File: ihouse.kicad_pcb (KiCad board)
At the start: 2 copper layers, 42 parts, among them J1 Conn_01x01, J2 Conn_01x01, J3 Conn_01x01, J4 Conn_01x01, J5 Conn_01x16, J6 Conn_01x02, J7 Conn_01x02, K1 FINDER-32.21-x300, K2 RT42xxxx, K3 FINDER-32.21-x300, K4 RT42xxxx, K5 G5Q-1A, K6 G5Q-1A, T1 Transformer_TEZ_22x24_6V, U1 LTV-817, U3 MOC3060S, U4 LTV-817, U5 MOC3060S

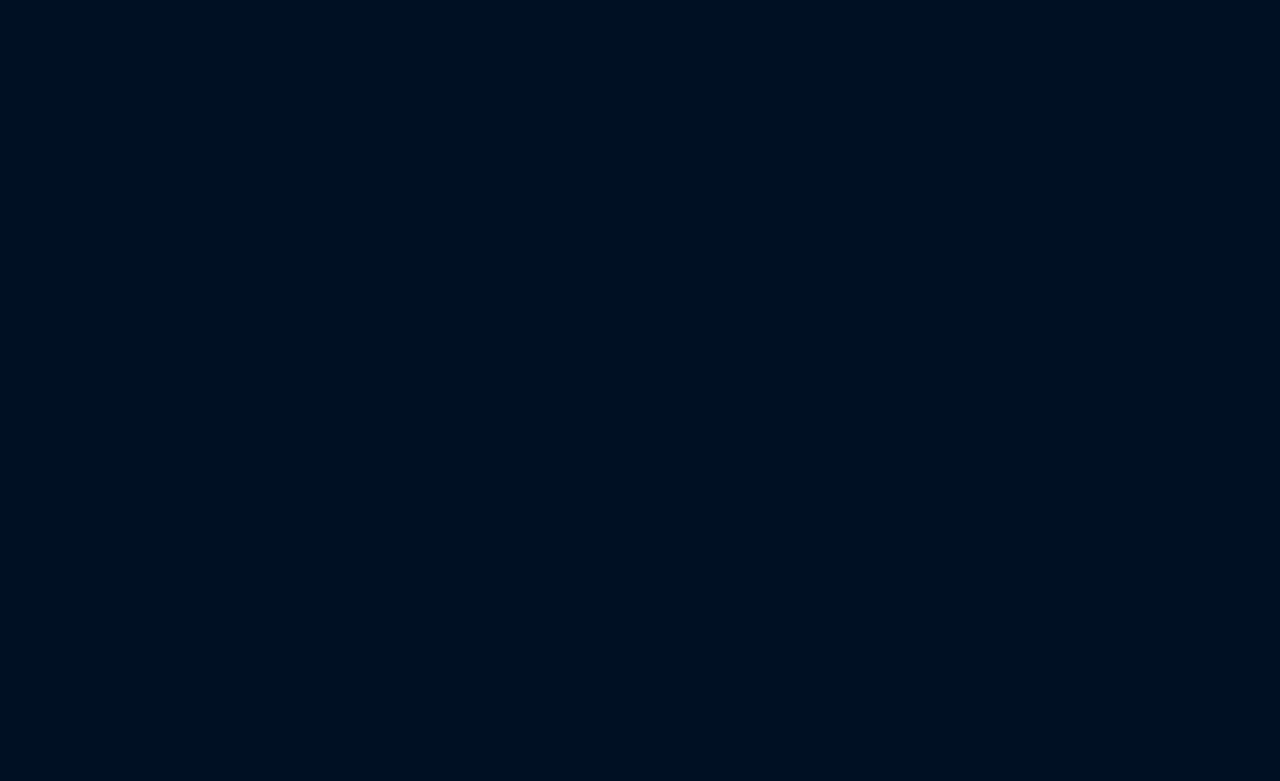
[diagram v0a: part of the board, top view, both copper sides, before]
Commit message: schemos paruosimas
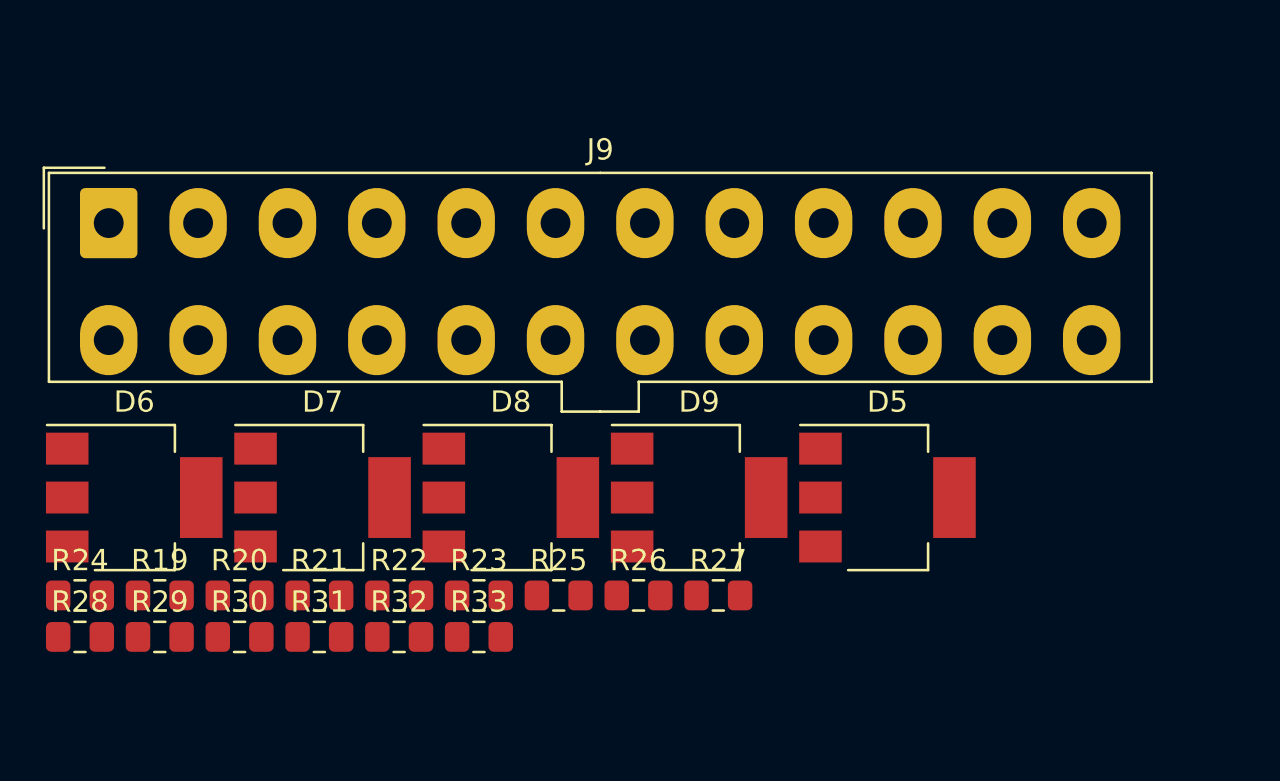
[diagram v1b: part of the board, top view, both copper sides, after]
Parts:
- added D5: Z0103MN, Package_TO_SOT_SMD:SOT-223, F.Cu at (71.6, 121.1)
- added D6: Z0103MN, Package_TO_SOT_SMD:SOT-223, F.Cu at (36.2, 121.1)
- added D7: Z0103MN, Package_TO_SOT_SMD:SOT-223, F.Cu at (45.0, 121.1)
- added D8: Z0103MN, Package_TO_SOT_SMD:SOT-223, F.Cu at (53.9, 121.1)
- added D9: Z0103MN, Package_TO_SOT_SMD:SOT-223, F.Cu at (62.7, 121.1)
- added J9: Conn_01x24, Connector_Molex:Molex_Mini-Fit_Jr_5566-24A_2x12_P4.20mm_Vertical, F.Cu at (35.0, 108.2)
- added R19: R, Resistor_SMD:R_0805_2012Metric_Pad1.15x1.40mm_HandSolder, F.Cu at (37.4, 125.7)
- added R20: R, Resistor_SMD:R_0805_2012Metric_Pad1.15x1.40mm_HandSolder, F.Cu at (41.1, 125.7)
- added R21: R, Resistor_SMD:R_0805_2012Metric_Pad1.15x1.40mm_HandSolder, F.Cu at (44.9, 125.7)
- added R22: R, Resistor_SMD:R_0805_2012Metric_Pad1.15x1.40mm_HandSolder, F.Cu at (48.6, 125.7)
- added R23: R, Resistor_SMD:R_0805_2012Metric_Pad1.15x1.40mm_HandSolder, F.Cu at (52.4, 125.7)
- added R24: R, Resistor_SMD:R_0805_2012Metric_Pad1.15x1.40mm_HandSolder, F.Cu at (33.6, 125.7)
- added R25: R, Resistor_SMD:R_0805_2012Metric_Pad1.15x1.40mm_HandSolder, F.Cu at (56.1, 125.7)
- added R26: R, Resistor_SMD:R_0805_2012Metric_Pad1.15x1.40mm_HandSolder, F.Cu at (59.9, 125.7)
- added R27: R, Resistor_SMD:R_0805_2012Metric_Pad1.15x1.40mm_HandSolder, F.Cu at (63.6, 125.7)
- added R28: R, Resistor_SMD:R_0805_2012Metric_Pad1.15x1.40mm_HandSolder, F.Cu at (33.6, 127.6)
- added R29: R, Resistor_SMD:R_0805_2012Metric_Pad1.15x1.40mm_HandSolder, F.Cu at (37.4, 127.6)
- added R30: R, Resistor_SMD:R_0805_2012Metric_Pad1.15x1.40mm_HandSolder, F.Cu at (41.1, 127.6)
- added R31: R, Resistor_SMD:R_0805_2012Metric_Pad1.15x1.40mm_HandSolder, F.Cu at (44.9, 127.6)
- added R32: R, Resistor_SMD:R_0805_2012Metric_Pad1.15x1.40mm_HandSolder, F.Cu at (48.6, 127.6)
- added R33: R, Resistor_SMD:R_0805_2012Metric_Pad1.15x1.40mm_HandSolder, F.Cu at (52.4, 127.6)
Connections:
- F1 pad 1: (no net) -> Net-(F1-Pad1)
- J5 pad 10: /EXTWC_L -> /EHALLIT_N
- J5 pad 11: /EHALLIT_N -> /WRKLIT_L
- J5 pad 12: (no net) -> /EHALLIT_N
- J5 pad 13: /EHALLIT_N -> /EHALLIT_L
- J5 pad 14: (no net) -> /EHALLIT_N
- J5 pad 15: /EHALLIT_N -> Net-(J5-Pad15)
- J5 pad 16: (no net) -> Net-(J5-Pad16)
- J5 pad 5: /230VAC_N -> /230VAC_L
- J5 pad 6: /230VAC_L -> /PE
- J5 pad 7: /230VAC_L -> /EXTKITCH_L
- J5 pad 8: /EXTKITCH_L -> /EHALLIT_N
- J5 pad 9: /EHALLIT_N -> /EXTWC_L
- K2 pad 12: (no net) -> Net-(K2-Pad12)
- K2 pad A1: (no net) -> /Power outputs/K0
- K4 pad 11: (no net) -> /ISOCK_N
- K4 pad 12: (no net) -> Net-(K4-Pad12)
- K4 pad 21: (no net) -> /ISOCK_L
- K4 pad 22: (no net) -> Net-(K4-Pad22)
- K4 pad A1: (no net) -> /Power outputs/K1
- R1 pad 1: (no net) -> /Controller/VREF
- R11 pad 1: (no net) -> Net-(D2-Pad3)
- U1 pad 4: (no net) -> /Controller/LPULSE
- U3 pad 2: (no net) -> /Power outputs/OC1
- U3 pad 3: (no net) -> Net-(U3-Pad3)
- U3 pad 5: (no net) -> Net-(U3-Pad5)
- U4 pad 3: (no net) -> /Power outputs/COM
- U4 pad 4: (no net) -> /Power outputs/LIGHTON
- U5 pad 2: (no net) -> /Power outputs/OC2
- U5 pad 3: (no net) -> Net-(U5-Pad3)
- U5 pad 5: (no net) -> Net-(U5-Pad5)

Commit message: tarpinis kommitas
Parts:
- moved T1 342.6 mm to (480.5, -25.2)
- moved D1 342.6 mm to (453.7, 21.3)
- moved D2 342.6 mm to (453.7, 23.6)
- moved D3 342.6 mm to (465.3, 17.9)
- moved D5 342.6 mm to (398.4, 18.4)
- moved D6 342.6 mm to (363.0, 18.4)
- moved D8 342.6 mm to (380.7, 18.4)
- moved F1 342.6 mm to (426.6, 19.6)
- moved J1 342.6 mm to (441.4, -76.4)
- moved J2 342.6 mm to (441.4, -73.7)
- moved J4 342.6 mm to (441.4, -71.1)
- moved J7 342.6 mm to (493.4, -64.8)
- moved K1 342.6 mm to (406.9, -22.4)
- moved K2 342.6 mm to (406.9, -16.8)
- moved R1 342.6 mm to (497.5, 0.59)
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
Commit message: tarpinis kommitas
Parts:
- removed D1: LL4148, Diode_SMD:D_MiniMELF
- removed D2: Z0103MN, Diode_SMD:D_MiniMELF
- removed D3: LL4148, Package_TO_SOT_SMD:SOT-223
- removed D4, D5, D6, D7, D8, D9: Z0103MN, Package_TO_SOT_SMD:SOT-223
- removed F1: 3A, Fuse:Fuseholder_Cylinder-5x20mm_Schurter_0031_8201_Horizontal_Open
- removed J1, J2: Conn_01x01, mech:Faston_6.3x0.8x14
- removed J9: Conn_01x24, Connector_Molex:Molex_Mini-Fit_Jr_5566-24A_2x12_P4.20mm_Vertical
- removed K1: FINDER-32.21-x300, Relay_THT:Relay_SPDT_Finder_34.51_Vertical
- removed K2: RT42xxxx, Relay_THT:Relay_SPDT_Finder_34.51_Vertical
- removed K3: FINDER-32.21-x300, Relay_THT:Relay_DPDT_Schrack-RT2-FormC_RM5mm
- removed K4: RT42xxxx, Relay_THT:Relay_DPDT_Schrack-RT2-FormC_RM5mm
- removed K5, K6: G5Q-1A, Relay_THT:Relay_SPST_Schrack-RT1-FormA_RM5mm
- removed R1, R2: Rx, Resistor_SMD:R_0805_2012Metric_Pad1.15x1.40mm_HandSolder
- removed R10, R11: R, Resistor_SMD:R_1206_3216Metric_Pad1.42x1.75mm_HandSolder
- removed R12, R15: 33k, Resistor_SMD:R_0805_2012Metric_Pad1.15x1.40mm_HandSolder
- removed R13, R14, R5, R6, R7, R8: 33k, Resistor_SMD:R_1206_3216Metric_Pad1.42x1.75mm_HandSolder
- removed R16, R17, R18, R19, R20, R21, R22, R23, R24, R25, R26, R27, R28, R29, R30, R31, R32, R33, R9: R, Resistor_SMD:R_0805_2012Metric_Pad1.15x1.40mm_HandSolder
- removed R3: 120, Resistor_SMD:R_0805_2012Metric_Pad1.15x1.40mm_HandSolder
- removed R4: 1k, Resistor_SMD:R_0805_2012Metric_Pad1.15x1.40mm_HandSolder
- removed T1: Transformer_TEZ_22x24_6V, Transformer_THT:Transformer_Breve_TEZ-22x24
- removed U1: LTV-817, Package_DIP:DIP-4_W7.62mm
- removed U3: MOC3060S, disc:DIP-6_W9.53mm_SMD
- removed U4: LTV-817, disc:DIP-6_W9.53mm_SMD
- added C10: 0.1, Capacitors_SMD:C_0805, F.Cu at (197.0, 35.2)
- added C11: 0.1, Capacitors_SMD:C_0805, F.Cu at (195.2, 39.9)
- added C2: 0.1, Capacitors_SMD:C_0805, F.Cu at (69.9, 84.8)
- added C3: 0.1, Capacitors_SMD:C_0805, F.Cu at (64.8, 99.6)
- added C4: 0.1, Capacitors_SMD:C_0805, F.Cu at (66.0, 95.5)
- added C5: 0.1, Capacitors_SMD:C_0805, F.Cu at (194.2, 33.4)
- added C6: 0.1, Capacitors_SMD:C_0805, F.Cu at (191.7, 39.9)
- added C7: 0.1, Capacitors_SMD:C_0805, F.Cu at (197.8, 33.4)
- added C8: 0.1, Capacitors_SMD:C_0805, F.Cu at (97.4, 78.4)
- added C9: 0.1, Capacitors_SMD:C_0805, F.Cu at (201.3, 33.4)
- added D13: D, Diodes_SMD:D_MiniMELF, F.Cu at (42.3, 99.3)
- added D14: D, Diodes_SMD:D_MiniMELF, F.Cu at (192.6, 35.6)
- added D15: D, Diodes_SMD:D_MiniMELF, F.Cu at (188.2, 40.0)
- added D16: D, Diodes_SMD:D_MiniMELF, F.Cu at (88.6, 85.0)
- added D17: D, Diodes_SMD:D_MiniMELF, F.Cu at (47.6, 99.3)
- added J12: Valves, Connectors_Molex:Molex_MiniFit-JR-5556-10A_2x05x4.20mm_Straight, F.Cu at (228.0, 122.0)
- added J13: Conn_01x04, Connectors_Molex:Molex_KK-6410-04_04x2.54mm_Straight, F.Cu at (232.0, 53.0)
- added J14: Conn_01x04, Connectors_Molex:Molex_KK-6410-04_04x2.54mm_Straight, F.Cu at (232.0, 64.0)
- added J15: Conn_01x04, Connectors_Molex:Molex_KK-6410-04_04x2.54mm_Straight, F.Cu at (232.0, 75.0)
- added J16: Conn_01x04, Connectors_Molex:Molex_KK-6410-04_04x2.54mm_Straight, F.Cu at (232.0, 86.0)
- added K10: FINDER-34.51, Relays_THT:Relay_SPDT_SingleRow_Standing_FinderType34Point51, F.Cu at (181.5, 136.0)
- added K11: FINDER-34.51, Relays_THT:Relay_SPDT_SingleRow_Standing_FinderType34Point51, F.Cu at (187.5, 136.0)
- added K12: RT42xxxx, Relays_THT:Relay_DPDT_Schrack-RT2-FormC_RM5mm, F.Cu at (194.7, 116.4)
- added K13: RT42xxxx, Relays_THT:Relay_DPDT_Schrack-RT2-FormC_RM5mm, F.Cu at (194.7, 130.9)
- added K14: FINDER-34.51, Relays_THT:Relay_SPDT_SingleRow_Standing_FinderType34Point51, F.Cu at (190.0, 89.0)
- added K15: FINDER-34.51, Relays_THT:Relay_SPDT_SingleRow_Standing_FinderType34Point51, F.Cu at (184.0, 89.0)
- added K16: RT42xxxx, Relays_THT:Relay_DPDT_Schrack-RT2-FormC_RM5mm, F.Cu at (194.7, 86.5)
- added K17: RT42xxxx, Relays_THT:Relay_DPDT_Schrack-RT2-FormC_RM5mm, F.Cu at (194.7, 101.0)
- added R43: R, Resistors_SMD:R_0805, F.Cu at (97.2, 80.3)
- added R44: R, Resistors_SMD:R_0805, F.Cu at (196.8, 37.0)
- added R45: R, Resistors_SMD:R_0805, F.Cu at (173.0, 71.0)
- added R46: R, Resistors_SMD:R_0805, F.Cu at (173.0, 74.0)
- added R47: R, Resistors_SMD:R_0805, F.Cu at (173.0, 77.0)
- added R48: R, Resistors_SMD:R_0805, F.Cu at (173.0, 81.0)
- added R49: R, Resistors_SMD:R_0805, F.Cu at (205.5, 32.3)
- added R50: R, Resistors_SMD:R_0805, F.Cu at (189.0, 55.0)
- added R51: R, Resistors_SMD:R_0805, F.Cu at (189.0, 51.0)
- added R52: R, Resistors_SMD:R_0805, F.Cu at (189.0, 59.0)
- added R53: R, Resistors_SMD:R_0805, F.Cu at (189.0, 63.0)
- added R54: R, Resistors_SMD:R_0805, F.Cu at (189.0, 72.0)
- added R55: R, Resistors_SMD:R_0805, F.Cu at (189.0, 74.0)
- added R56: R, Resistors_SMD:R_0805, F.Cu at (189.0, 76.0)
- added R57: R, Resistors_SMD:R_0805, F.Cu at (192.0, 76.0)
- added RN1: R_Pack04, Resistors_SMD:R_Array_Convex_4x1206, F.Cu at (98.9, 67.6)
- added RN2: R_Pack04, Resistors_SMD:R_Array_Convex_4x1206, F.Cu at (198.0, 64.0)
- added RN3: R_Pack04, Resistors_SMD:R_Array_Convex_4x1206, F.Cu at (97.8, 74.6)
- added RN4: R_Pack04, Resistors_SMD:R_Array_Convex_4x1206, F.Cu at (211.0, 62.0)
- added U10: MOC3060S, disc:DIP-6_W9.53mm_SMD, F.Cu at (85.6, -77.9)
- added U11: MOC3060S, disc:DIP-6_W9.53mm_SMD, F.Cu at (73.4, -61.4)
- added U12: MOC3060S, disc:DIP-6_W9.53mm_SMD, F.Cu at (85.6, -69.6)
- added U13: MOC3060S, disc:DIP-6_W9.53mm_SMD, F.Cu at (97.9, -77.9)
- added U14: MOC3060S, disc:DIP-6_W9.53mm_SMD, F.Cu at (85.6, -61.4)
- added U16: ULN2803A, Housings_SOIC:SOIC-18W_7.5x11.6mm_Pitch1.27mm, F.Cu at (151.0, 110.0)
- added U6: MOC3060S, disc:DIP-6_W9.53mm_SMD, F.Cu at (61.1, -69.6)
- added U7: MOC3060S, disc:DIP-6_W9.53mm_SMD, F.Cu at (73.4, -77.9)
- added U8: MOC3060S, disc:DIP-6_W9.53mm_SMD, F.Cu at (61.1, -61.4)
- added U9: MOC3060S, disc:DIP-6_W9.53mm_SMD, F.Cu at (73.4, -69.6)
- J5: value Conn_01x16 -> Conn_01x01; footprint Connectors_Phoenix:PhoenixContact_MSTBA-G_16x5.00mm_Angled -> mech:Faston_6.3x0.8x14
- J6: value Conn_01x02 -> Conn_01x01; footprint Connectors_Phoenix:PhoenixContact_MSTBA-G_02x5.00mm_Angled -> mech:Faston_6.3x0.8x14
- J7: value Conn_01x02 -> Conn_01x03; footprint Connectors_Phoenix:PhoenixContact_MSTBA-G_02x5.00mm_Angled -> Connectors_Phoenix:PhoenixContact_MSTBA-G_03x5.00mm_Angled
- moved J5 420.6 mm to (123.3, -67.2), turned to 0 degrees
- moved J7 380.3 mm to (113.3, -79.1)
- moved J6 348.7 mm to (131.9, -78.0)
- moved J3 337.0 mm to (113.9, -67.2)
- moved U5 330.6 mm to (61.1, -77.9)
- moved C1 318.7 mm to (59.7, -46.7)
- moved J4 309.6 mm to (131.9, -80.7)
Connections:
- J5 pad 1: /230VAC_L -> /PE
- J6 pad 1: /Power outputs/LIGHTBASH1 -> /PE
- J7 pad 1: /Power outputs/LIGHTWC1 -> /230VAC_L
- J7 pad 2: /Power outputs/LIGHTWC2 -> /230VAC_N
- U5 pad 2: /Power outputs/OC2 -> /Power outputs/OC1
- U5 pad 4: /EXTKITCH_L -> /Power outputs/OUTAC9
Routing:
- net /DC sklendziu valdymas/12VDC: track 0.00 -> 111.7 mm, vias 0 -> 2
- net /DC sklendziu valdymas/V3A2: track 0.00 -> 56.1 mm
- net /DC sklendziu valdymas/V3TST: track 0.00 -> 51.3 mm, vias 0 -> 4
- net /DC sklendziu valdymas/V2TST: track 0.00 -> 50.3 mm, vias 0 -> 2
- net /DC sklendziu valdymas/V1TST: track 0.00 -> 47.6 mm, vias 0 -> 2
- net /DC sklendziu valdymas/V4A2: track 0.00 -> 47.4 mm, vias 0 -> 2
- net /DC sklendziu valdymas/V4TST: track 0.00 -> 43.6 mm, vias 0 -> 2
- net /DC sklendziu valdymas/V2A1: track 0.00 -> 32.7 mm, vias 0 -> 2
- net /DC sklendziu valdymas/V3A1: track 0.00 -> 31.8 mm, vias 0 -> 2
- net /DC sklendziu valdymas/V2A2: track 0.00 -> 28.4 mm
- net /DC sklendziu valdymas/V1A2: track 0.00 -> 19.5 mm
- net /DC sklendziu valdymas/V4A1: track 0.00 -> 16.9 mm
- net /DC sklendziu valdymas/V1A1: track 0.00 -> 15.5 mm
- added copper zone on B.Cu, net /DC sklendziu valdymas/COM
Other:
- board outline added: 64 x 94 mm

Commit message: tarpinis kommitas
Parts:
- removed C1: 100uFx16V, Capacitors_SMD:CP_Elec_6.3x5.7
- removed C10, C11, C2, C3, C4, C5, C6, C7, C8, C9: 0.1, Capacitors_SMD:C_0805
- removed D13, D14, D15, D16, D17: D, Diodes_SMD:D_MiniMELF
- removed J12: Valves, Connectors_Molex:Molex_MiniFit-JR-5556-10A_2x05x4.20mm_Straight
- removed J13, J14, J15, J16: Conn_01x04, Connectors_Molex:Molex_KK-6410-04_04x2.54mm_Straight
- removed J3, J4, J5, J6: Conn_01x01, mech:Faston_6.3x0.8x14
- removed J7: Conn_01x03, Connectors_Phoenix:PhoenixContact_MSTBA-G_03x5.00mm_Angled
- removed K10, K11, K14, K15: FINDER-34.51, Relays_THT:Relay_SPDT_SingleRow_Standing_FinderType34Point51
- removed K12, K13, K16, K17: RT42xxxx, Relays_THT:Relay_DPDT_Schrack-RT2-FormC_RM5mm
- removed R43, R44, R45, R46, R47, R48, R49, R50, R51, R52, R53, R54, R55, R56, R57: R, Resistors_SMD:R_0805
- removed RN1, RN2, RN3, RN4: R_Pack04, Resistors_SMD:R_Array_Convex_4x1206
- removed U10, U11, U12, U13, U14, U5, U6, U7, U8, U9: MOC3060S, disc:DIP-6_W9.53mm_SMD
- removed U16: ULN2803A, Housings_SOIC:SOIC-18W_7.5x11.6mm_Pitch1.27mm
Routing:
- net /DC sklendziu valdymas/12VDC: track 111.7 -> 0.00 mm, vias 2 -> 0
- net /DC sklendziu valdymas/V3A2: track 56.1 -> 0.00 mm
- net /DC sklendziu valdymas/V3TST: track 51.3 -> 0.00 mm, vias 4 -> 0
- net /DC sklendziu valdymas/V2TST: track 50.3 -> 0.00 mm, vias 2 -> 0
- net /DC sklendziu valdymas/V1TST: track 47.6 -> 0.00 mm, vias 2 -> 0
- net /DC sklendziu valdymas/V4A2: track 47.4 -> 0.00 mm, vias 2 -> 0
- net /DC sklendziu valdymas/V4TST: track 43.6 -> 0.00 mm, vias 2 -> 0
- net /DC sklendziu valdymas/V2A1: track 32.7 -> 0.00 mm, vias 2 -> 0
- net /DC sklendziu valdymas/V3A1: track 31.8 -> 0.00 mm, vias 2 -> 0
- net /DC sklendziu valdymas/V2A2: track 28.4 -> 0.00 mm
- net /DC sklendziu valdymas/V1A2: track 19.5 -> 0.00 mm
- net /DC sklendziu valdymas/V4A1: track 16.9 -> 0.00 mm
- net /DC sklendziu valdymas/V1A1: track 15.5 -> 0.00 mm
- removed copper zone on B.Cu, net /DC sklendziu valdymas/COM
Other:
- board outline removed
